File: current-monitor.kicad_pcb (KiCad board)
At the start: 2 copper layers, 91 parts, among them J103 USB-MICROB, J501 JTAG, U201 AD8429A, U202 LM833, U203 TL032C, U301 INA826, U401 LM27313, U402 LTC3260MSE, U403 MAX6070, U501 K22F-64LQFP, U601 TL032C

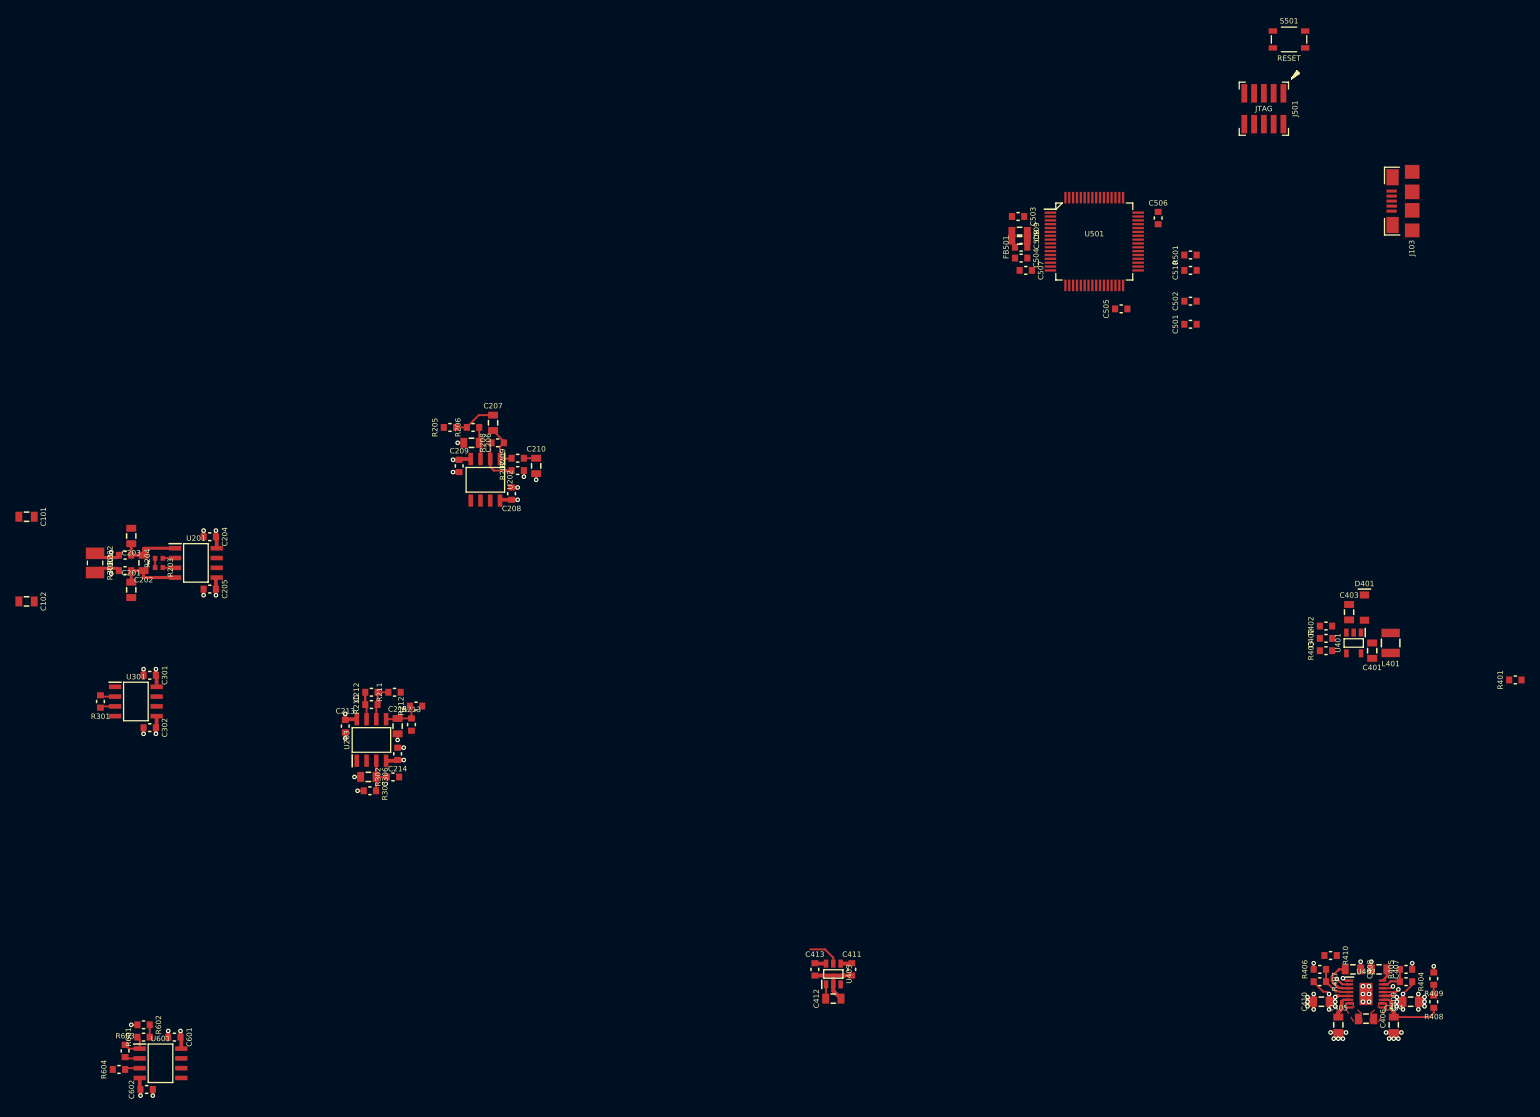
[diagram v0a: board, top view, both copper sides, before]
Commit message: more layout
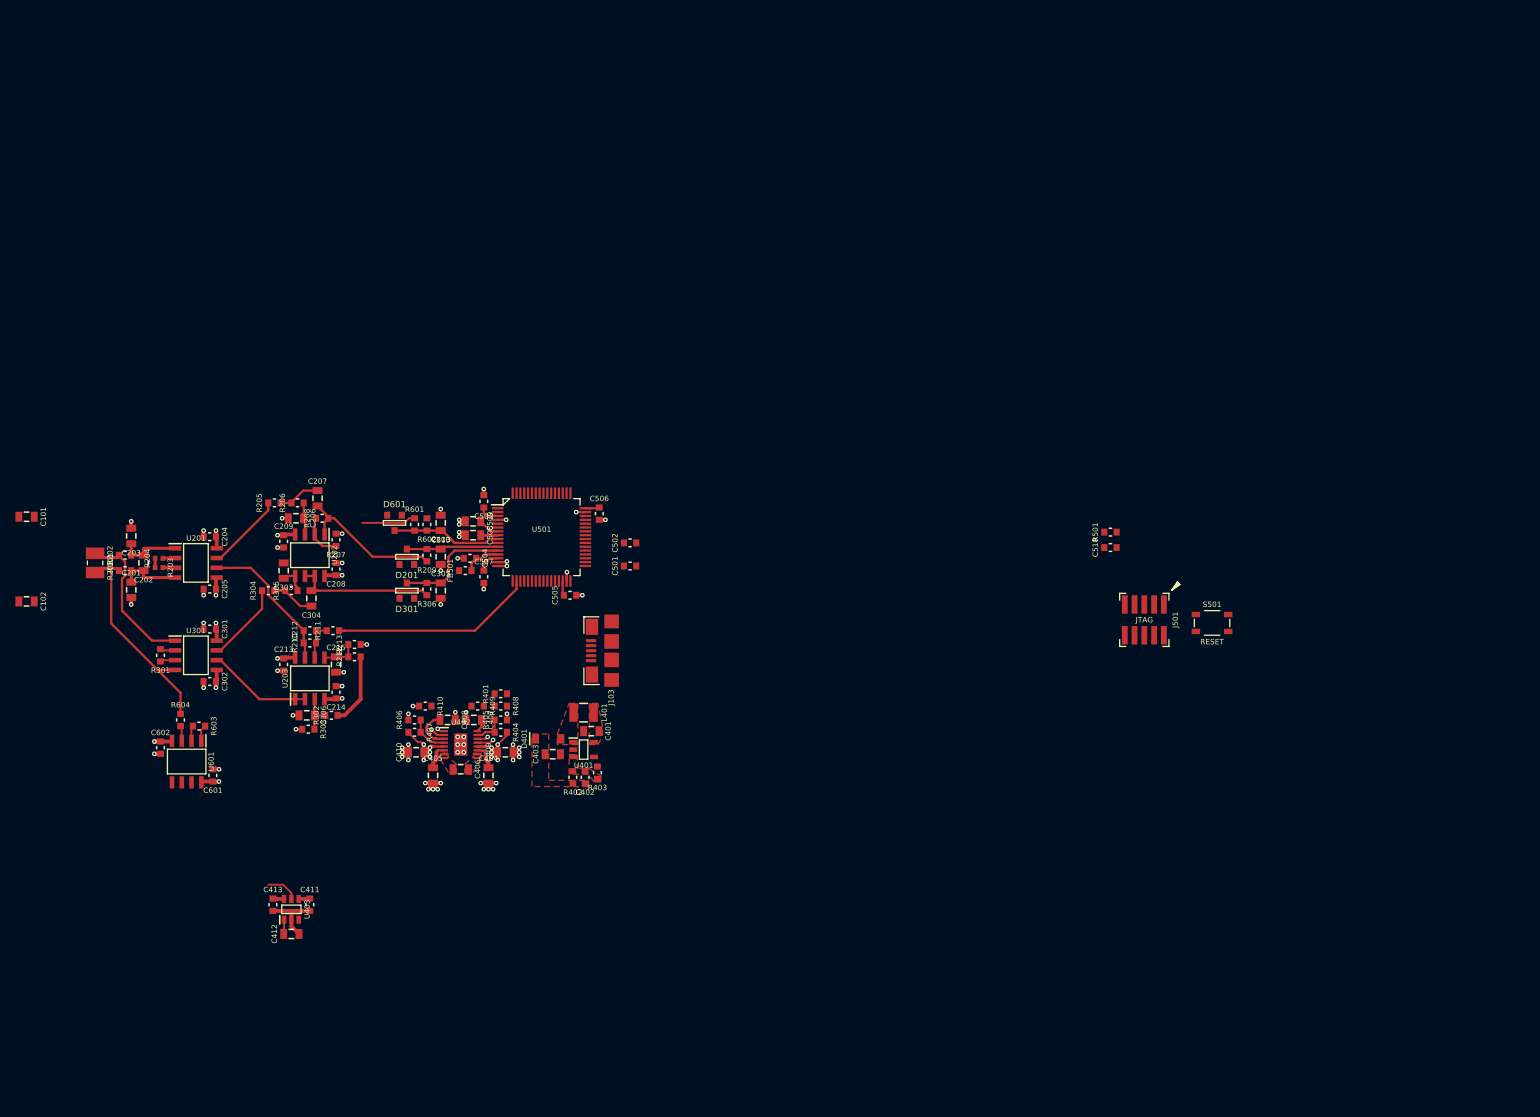
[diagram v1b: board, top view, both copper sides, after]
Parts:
- added C303: C, libs:SMD-2012, F.Cu at (112.4, 86.0)
- added C304: C, libs:SMD-2012, F.Cu at (116.0, 89.6)
- added C305: C, libs:SMD-2012, F.Cu at (132.8, 88.6)
- added C603: 4n, libs:SMD-2012, F.Cu at (132.8, 79.8)
- added D201: BAS40-04, libs:SOT-23, F.Cu at (128.4, 84.2)
- added D301: BAS40-04, libs:SOT-23, F.Cu at (128.4, 88.6)
- added D601: BAS40-04, libs:SOT-23, F.Cu at (126.8, 79.8)
- added R304: Rs, libs:SMD-1608, F.Cu at (110.4, 88.6)
- added R305: Rs, libs:SMD-1608, F.Cu at (113.4, 88.6)
- added R306: R, libs:SMD-1608, F.Cu at (131.0, 88.4)
- moved R401 131.8 mm to (140.6, 102.0)
- moved R409 129.1 mm to (137.6, 103.6), turned to 270 degrees
- moved R408 127.1 mm to (140.6, 103.6), turned to 270 degrees
- moved C404 122.0 mm to (139.0, 112.6)
- moved C408 122.0 mm to (133.7, 105.4)
- moved C409 122.0 mm to (141.2, 109.6)
- moved C405 122.0 mm to (131.8, 112.6)
- moved C407 122.0 mm to (137.1, 105.4)
- moved C410 122.0 mm to (129.6, 109.6)
- moved R404 122.0 mm to (140.6, 107.0)
- moved R405 122.0 mm to (140.6, 105.4)
- moved R406 122.0 mm to (129.4, 105.4)
- moved R407 122.0 mm to (129.4, 107.0)
- moved R410 122.0 mm to (130.8, 103.6)
- moved U402 122.0 mm to (135.4, 108.6)
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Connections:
- net Net-(C207-Pad2) renamed /Current Sense Fine Range/FINE_UNCLAMPED
- net Net-(R601-Pad1) renamed /Sense Voltage/VOLTAGE_RAW
- U202 pad 5: (no net) -> Net-(C303-Pad1)
- U202 pad 6: (no net) -> /Current Sense Coarse Range/COARSE_UNCLAMPED
- U202 pad 7: (no net) -> /Current Sense Coarse Range/COARSE_UNCLAMPED
- U301 pad 7: /Current Sense Coarse Range/SENSE_COARSE -> Net-(R304-Pad1)
- U501 pad 10: /Current Sense Coarse Range/SENSE_COARSE -> (no net)
- U501 pad 11: /MCU/SENSE_VOLTAGE -> /Current Sense Fine Range/SENSE_FINE
- U501 pad 12: (no net) -> /Current Sense Coarse Range/SENSE_COARSE
- U501 pad 9: /Current Sense Fine Range/SENSE_FINE -> /MCU/SENSE_VOLTAGE
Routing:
- net /Current Sense Fine Range/REF_ADJUST: track 0.00 -> 26.3 mm
- net SENSE+: track 4.63 -> 28.8 mm, vias 1 -> 0
- net /Current Sense Coarse Range/COARSE_UNCLAMPED: track 0.00 -> 18.6 mm
- net COM: track 51.6 -> 68.8 mm, vias 48 -> 66
- net SENSE-: track 4.18 -> 19.6 mm, vias 1 -> 0
- net /Current Sense Fine Range/REF_FINE: track 5.07 -> 20.5 mm
- net /Current Sense Coarse Range/SENSE_COARSE: track 0.00 -> 15.1 mm
- net /MCU/SENSE_VOLTAGE: track 1.60 -> 16.5 mm
- net /Current Sense Fine Range/FINE_UNCLAMPED: track 5.99 -> 20.3 mm
- net /Current Sense Coarse Range/REF_COARSE: track 0.00 -> 13.6 mm
- net +3.00V: track 5.69 -> 18.0 mm
- net Net-(R304-Pad1): track 0.00 -> 10.5 mm
- net /Current Sense Fine Range/SENSE_FINE: track 1.60 -> 11.9 mm
- net Net-(R205-Pad1): track 0.00 -> 10.2 mm
- net +3V3: track 0.00 -> 9.16 mm
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- added copper zone on F.Cu, net +5V
- added copper zone on F.Cu, net /Power Supply/+Vs_UNREG
- added copper zone on F.Cu, net Net-(C402-Pad2)
- added copper zone on F.Cu, net Net-(D401-PadA)
